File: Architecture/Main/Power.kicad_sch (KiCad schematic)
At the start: 19 parts, among them J1 12V - Secteur, Q1 PMOS, Q2 NPN, U3 MIC2253

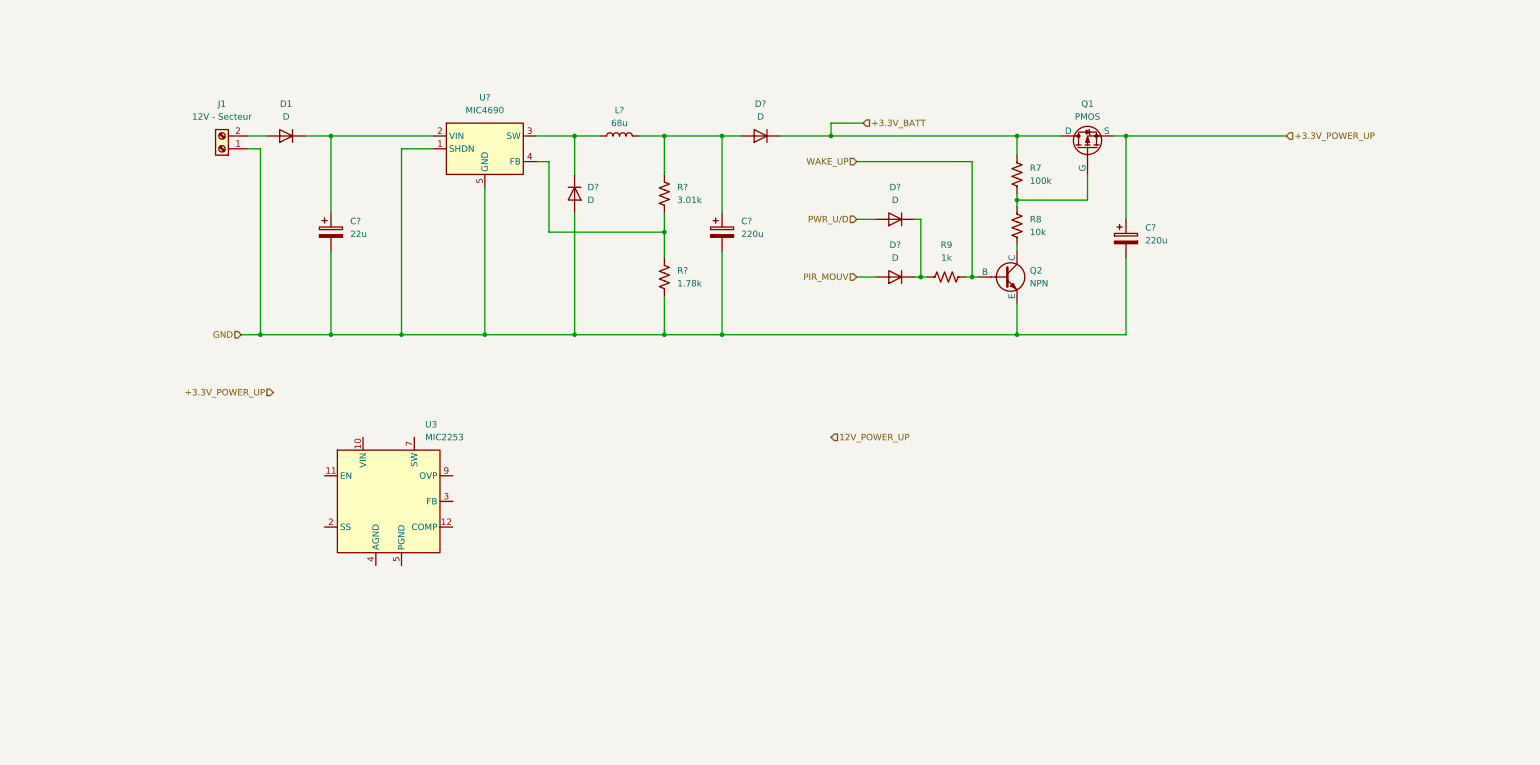
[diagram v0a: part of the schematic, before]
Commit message: Update_She
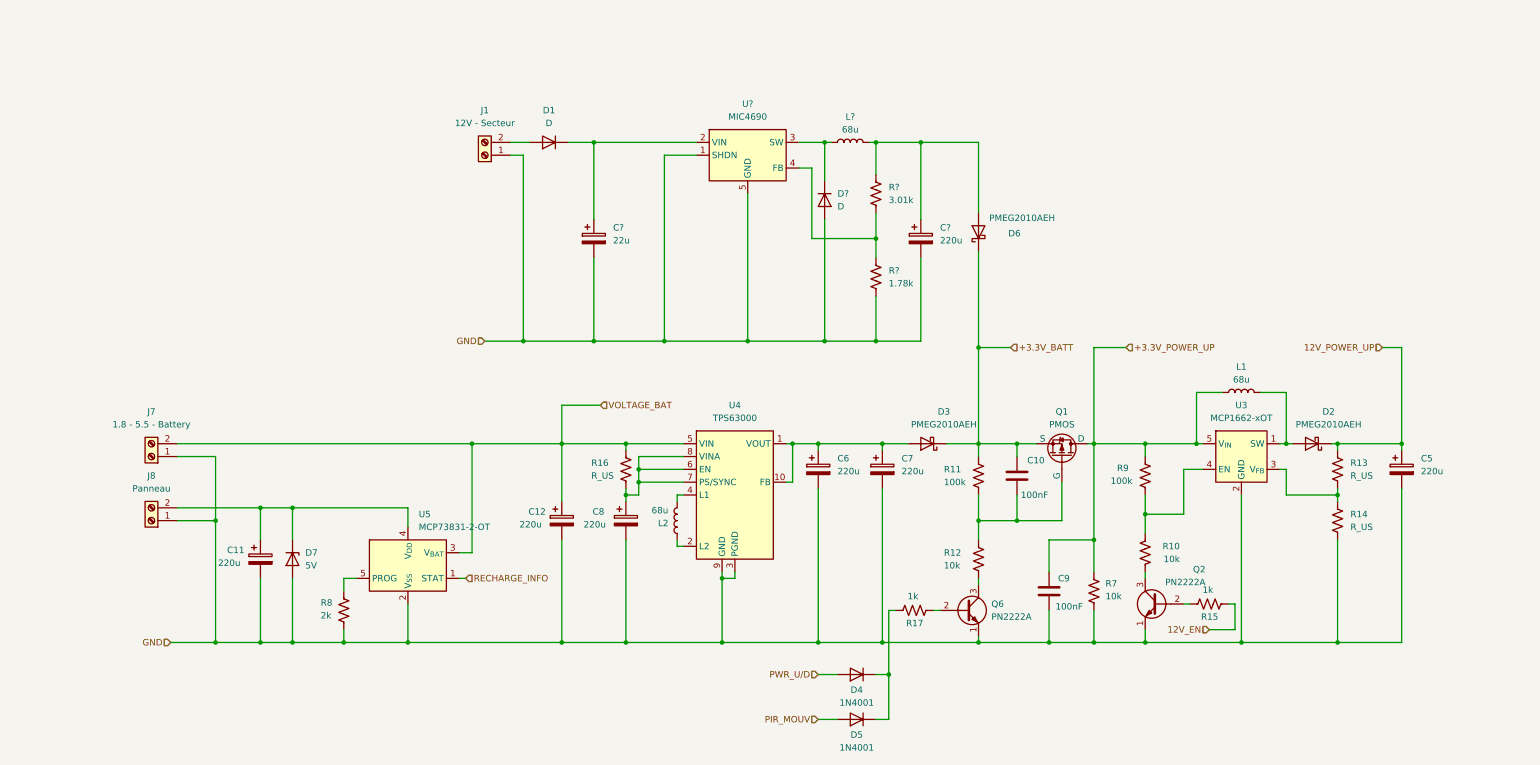
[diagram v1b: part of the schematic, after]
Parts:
- removed C?: 220u, symbol Device:C_Polarized
- removed D? (x3): D, symbol Device:D
- removed Q2: NPN, symbol Simulation_SPICE:NPN
- removed U3: MIC2253, Package_DFN_QFN:DFN-12-1EP_3x3mm_P0.5mm_EP1.6x2.5mm_ThermalVias, symbol Regulator_Switching:MIC2253
- added C10, C9: 100nF, symbol Device:C
- added C11, C12, C5, C6, C7, C8: 220u, symbol Device:C_Polarized
- added D2, D3, D6: PMEG2010AEH, Diode_SMD:D_SOD-123F, symbol Diode:PMEG2010AEH
- added D4, D5: 1N4001, Diode_THT:D_DO-41_SOD81_P10.16mm_Horizontal, symbol Diode:1N4001
- added D7: 5V, symbol Device:D_Zener
- added J7: 1.8 - 5.5 - Battery, symbol Connector:Screw_Terminal_01x02
- added J8: Panneau, symbol Connector:Screw_Terminal_01x02
- added L1, L2: 68u, symbol Device:L
- added Q2, Q6: PN2222A, Package_TO_SOT_THT:TO-92_Inline, symbol Transistor_BJT:PN2222A
- added R10, R12: 10k, symbol Device:R_US
- added R11: 100k, symbol Device:R_US
- added R13, R14, R16: R_US, symbol Device:R_US
- added R15, R17: 1k, symbol Device:R_US
- added U3: MCP1662-xOT, Package_TO_SOT_SMD:SOT-23-5, symbol Driver_LED:MCP1662-xOT
- added U4: TPS63000, Package_SON:Texas_DRC0010J_ThermalVias, symbol Regulator_Switching:TPS63000
- added U5: MCP73831-2-OT, Package_TO_SOT_SMD:SOT-23-5, symbol Battery_Management:MCP73831-2-OT
- R7: value 100k -> 10k; footprint Resistor_SMD:R_0805_2012Metric_Pad1.20x1.40mm_HandSolder -> (none)
- R8: value 10k -> 2k; footprint Resistor_SMD:R_0805_2012Metric_Pad1.20x1.40mm_HandSolder -> (none)
- R9: value 1k -> 100k; footprint Resistor_SMD:R_0805_2012Metric_Pad1.20x1.40mm_HandSolder -> (none)
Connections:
- net +3.3V_BATT: now also Q1.3 (S), C10.2, D3.1 (K), D6.1 (K), R11.1; no longer Q1.1 (D), R7.1
- net +3.3V_POWER_UP: now also Q1.1 (D), R7.1, R9.1, C9.1, L1.1, U3.5 (V_{IN}); no longer Q1.3 (S)
- net 12V_POWER_UP: now also C5.1, D2.1 (K), R13.1
- net GND: now also R7.2, R8.2, C11.2, C12.2, C5.2, C6.2, C7.2, C8.2, C9.2, D7.2 (A), J7.1 (Pin_1), J8.1 (Pin_1), Q2.1 (E), Q6.1 (E), R14.2, U3.2 (GND), U4.11 (PGND), U4.3 (PGND), U4.9 (GND), U5.2 (V_{SS})
- net PIR_MOUV: now also D5.2 (A)
- net PWR_U/D: now also D4.2 (A)
- net at C?.1, L?.2, R?.1: now also D6.2 (A)
- net WAKE_UP: no longer names the net of R9.2
- net WAKE_UP: now also R10.1, U3.4 (EN)
- new net: D4.1 (K), D5.1 (K), R17.1
- new net: Q6.2 (B), R17.2
- new net: C10.1, Q1.2 (G), R11.2, R12.1
- new net: Q2.3 (C), R10.2
- new net: C11.1, D7.1 (K), J8.2 (Pin_2), U5.4 (V_{DD})
- new net: R8.1, U5.5 (PROG)
- new net: C6.1, C7.1, D3.2 (A), U4.1 (VOUT), U4.10 (FB)
- new net: D2.2 (A), L1.2, U3.1 (SW)
- new net: Q2.2 (B), R15.1
- new net: L2.1, U4.2 (L2)
- new net: L2.2, U4.4 (L1)
- new net: C8.1, R16.2, U4.6 (EN), U4.7 (PS/SYNC), U4.8 (VINA)
- new net: R13.2, R14.1, U3.3 (V_{FB})
- new net: Q6.3 (C), R12.2
- new net 12V_EN: R15.2
- new net RECHARGE_INFO: U5.1 (STAT)
- new net VOLTAGE_BAT: C12.1, J7.2 (Pin_2), R16.1, U4.5 (VIN), U5.3 (V_{BAT})
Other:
- moved on the sheet: C?, D1, D?, J1, L?, R?, U?
